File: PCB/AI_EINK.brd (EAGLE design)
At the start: 66 x 111.6 mm, 184 parts, among them IC3 WM8960, J1 BM04B-GHS-TBT(LF)(SN)(N), J2 C393939, J3 524372471, Q1 SI1308EDL-T1-GE3, Q3 NMOS_C7465427, T1 MMUN2133LT1G, U1 TPS61090RSAR, U10 AP2112-3.3K, U11 AP2112-3.3K, U12 SPU0410LR5H-QB, U2 MC74VHC1G14DFT1G, U3 BQ27441DRZR-G1A, U4 BQ24075, U5 TLV74328, U6 TLV74315, U7 TLV74318PDBVRDBV0005A_L, U8 ST25DV64K-IER6S3SOIC_IER6S3_S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, U9 EMC2301-1-ACZL-TRMSOP8_MC_MCH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, Y1 ABM8-272-T3

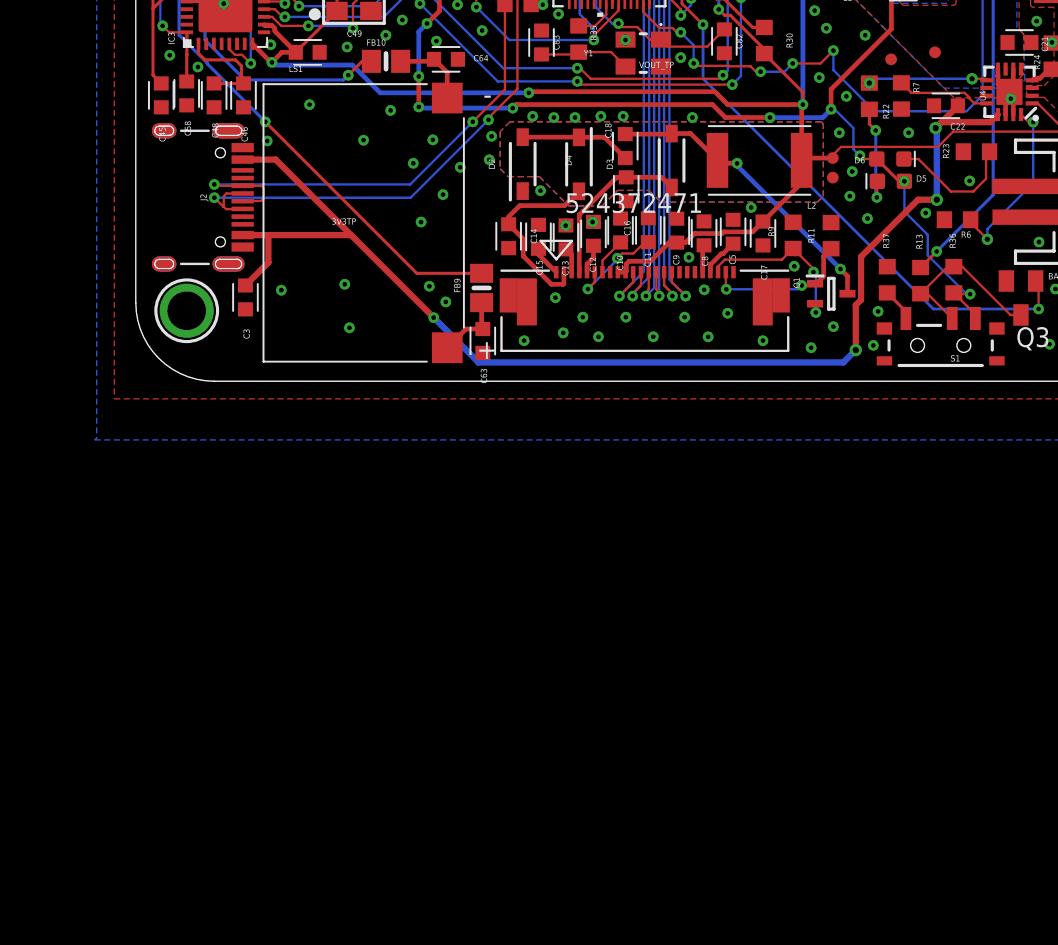
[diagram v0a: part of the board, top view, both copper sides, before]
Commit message: PCB
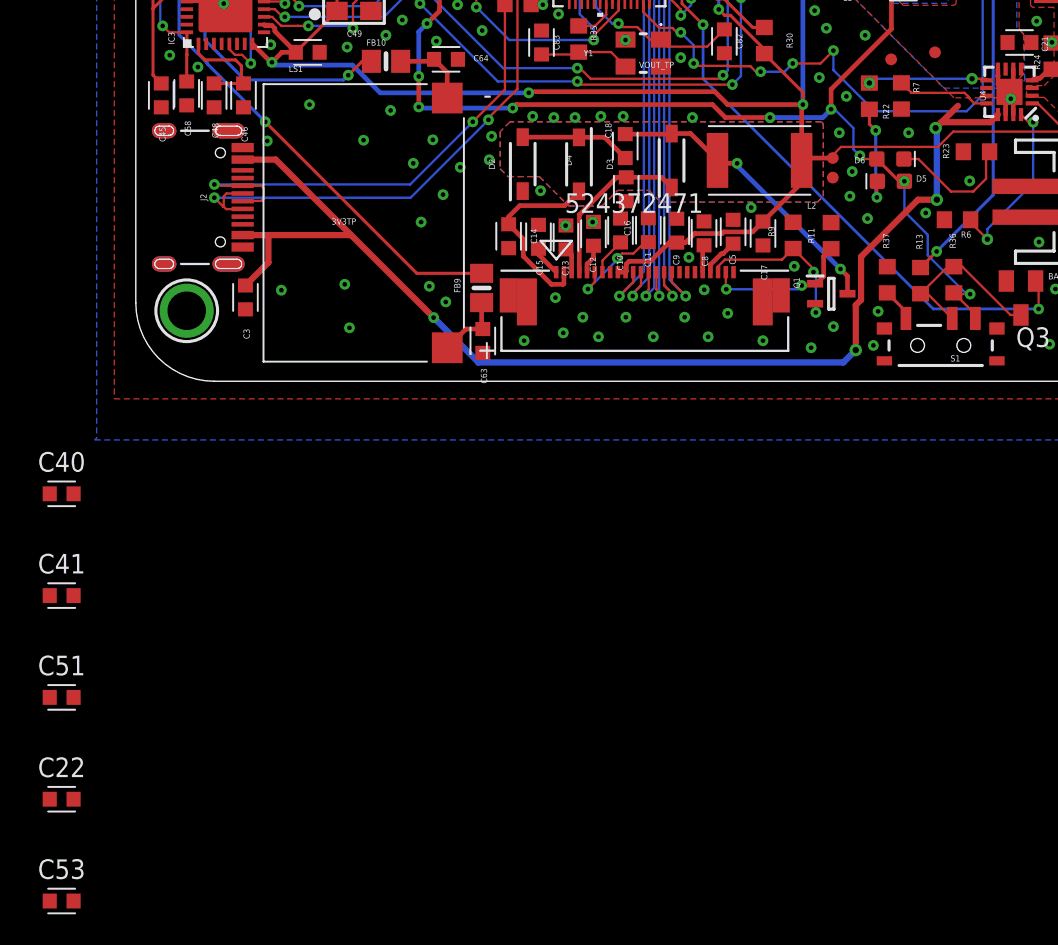
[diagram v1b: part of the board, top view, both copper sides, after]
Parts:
- added C40, C41, C51, C53: 10uF, Capacitor:CAPC1608X85
- C22: value 1.0uF -> 10uF
- moved C22 72.9 mm to (-3.81, -23.1), turned to 0 degrees
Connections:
- net GND: now also C40.2, C41.2, C51.2, C53.2
- net VBUS: now also C53.1
- net V_BATT: now also C40.1, C41.1, C51.1

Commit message: pcb before downsize
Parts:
- U1: value TPS61090RSAR -> TPS61092RSAR
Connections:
- new net N$20: RPI-CM1.29
- new net N$22: RPI-CM1.41
- new net N$28: RPI-CM1.55
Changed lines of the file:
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@@
 <attribute name="BOM" value="EXCLUDE" x="97.012" y="12.001" size="1.778" layer="27" display="off"/>
 </element>
-<element name="U1" library="microbuilder" package="PVQFN-16" value="TPS61090RSAR" x="53.434" y="35.658" smashed="yes">
+<element name="U1" library="microbuilder" package="PVQFN-16" value="TPS61092RSAR" x="53.434" y="35.658" smashed="yes">
 <attribute name="NAME" x="51.41" y="38.54" size="0.4064" layer="25" ratio="18"/>
 <attribute name="VALUE" x="51.31" y="32.418" size="0.4064" layer="27" ratio="10"/>
@@
 <contactref element="U8" pad="7"/>
 </signal>
+<signal name="N$20">
+<contactref element="RPI-CM1" pad="29"/>
+</signal>
+<signal name="N$22">
+<contactref element="RPI-CM1" pad="41"/>
+</signal>
+<signal name="N$28">
+<contactref element="RPI-CM1" pad="55"/>
+</signal>
 </signals>
